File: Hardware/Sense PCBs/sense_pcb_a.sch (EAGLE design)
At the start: 6 parts, among them J1 DF11-18DP-2DSA(24)

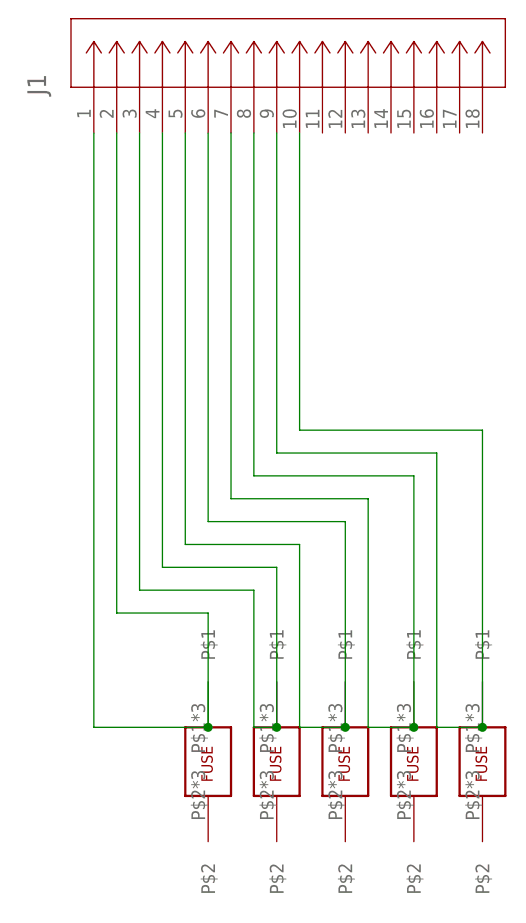
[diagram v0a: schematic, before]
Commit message: sense pcb a
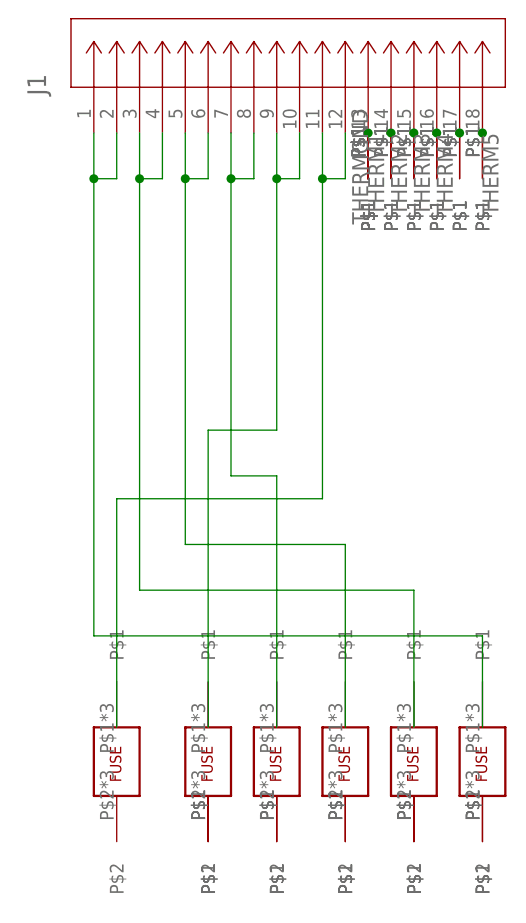
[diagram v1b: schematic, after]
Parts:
- added U$10, U$6, U$7, U$8, U$9: BB_CONTACT, sense_pcb_components:BB_CONTACT
- added U$11: FUSE, sense_pcb_components:FUSE
- added U$12, U$13, U$14, U$15, U$16, U$17, U$18, U$19, U$20, U$21, U$22, U$23, U$24, U$25, U$26, U$27, U$28, U$29, U$30, U$31: THERM_PIN, sense_pcb_components:THERM_PIN
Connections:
- new net N$11: J1.3, J1.4, U$4.P$1
- new net N$2: U$1.P$2, U$6.P$1
- new net N$4: U$2.P$2, U$7.P$1
- new net N$5: U$10.P$1, U$5.P$2
- new net N$6: U$3.P$2, U$8.P$1
- new net N$8: U$4.P$2, U$9.P$1
- new net THERM1: J1.14, U$22.P$1, U$23.P$1
- new net THERM2: J1.15, U$24.P$1, U$25.P$1
- new net THERM3: J1.16, U$26.P$1, U$27.P$1
- new net THERM4: J1.17, U$28.P$1, U$29.P$1
- new net THERM5: J1.18, U$30.P$1, U$31.P$1
- new net THERMGND: J1.13, U$12.P$1, U$13.P$1, U$14.P$1, U$15.P$1, U$16.P$1, U$17.P$1, U$18.P$1, U$19.P$1, U$20.P$1, U$21.P$1
- net N$1: now also J1.11, J1.12, U$11.P$1; no longer J1.1, J1.2, U$1.P$1
- net N$3: now also J1.1, J1.2, U$5.P$1; no longer J1.3, J1.4, U$2.P$1
- net N$7: now also J1.10, J1.9, U$1.P$1; no longer J1.7, J1.8, U$4.P$1
- net N$9: now also J1.7, J1.8, U$2.P$1; no longer J1.10, J1.9, U$5.P$1
